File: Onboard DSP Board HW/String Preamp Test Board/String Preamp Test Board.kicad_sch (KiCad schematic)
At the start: 27 parts, among them J1 Battery, J4 Output Jack, U1 TLV9002, U2 TP4054, U6 ${SIM.PARAMS}

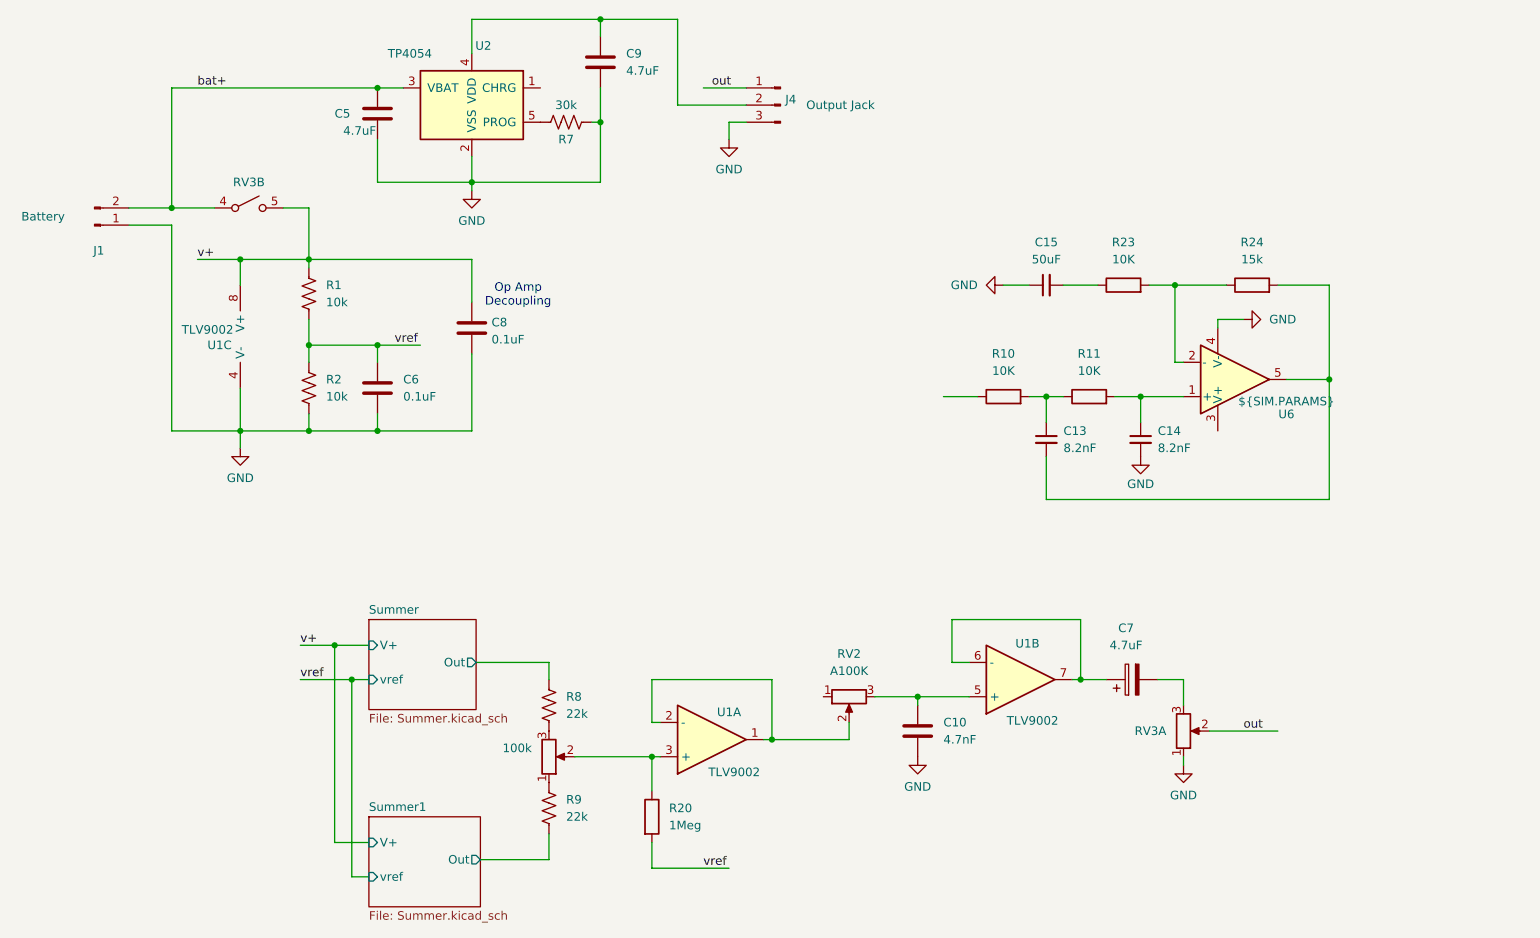
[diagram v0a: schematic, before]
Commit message: WIP
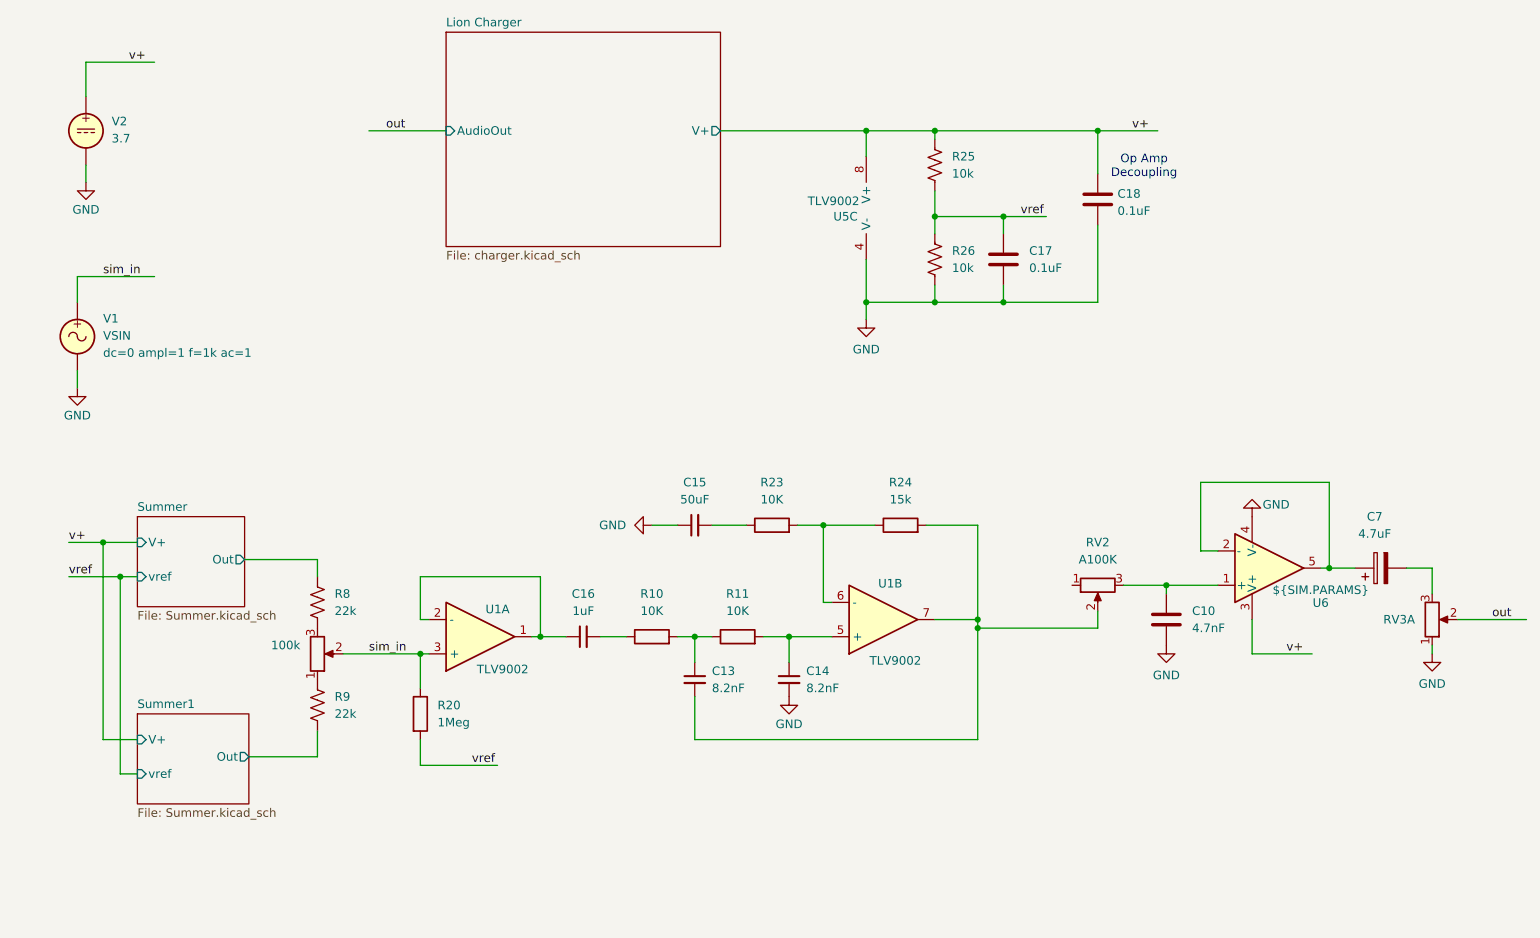
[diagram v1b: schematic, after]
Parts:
- removed C5, C9: 4.7uF, Capacitor_SMD:C_0603_1608Metric, symbol Device:C
- removed C6, C8: 0.1uF, Capacitor_SMD:C_0603_1608Metric, symbol Device:C
- removed J1: Battery, Connector_JST:JST_PH_S2B-PH-K_1x02_P2.00mm_Horizontal, symbol Connector:Conn_01x02_Male
- removed J4: Output Jack, Connector_PinHeader_2.54mm:PinHeader_1x03_P2.54mm_Vertical, symbol Connector:Conn_01x03_Male
- removed R1, R2: 10k, Resistor_SMD:R_0603_1608Metric, symbol Device:R_US
- removed R7: 30k, Resistor_SMD:R_0603_1608Metric, symbol Device:R_US
- removed unit 2 of RV3
- removed unit 3 of U1
- removed U2: TP4054, Package_TO_SOT_SMD:SOT-23-5, symbol Battery_Management:MCP73811T-420I-OT
- added C16: 1uF, symbol Device:C_Small
- added C17, C18: 0.1uF, Capacitor_SMD:C_0603_1608Metric, symbol Device:C
- added R25, R26: 10k, Resistor_SMD:R_0603_1608Metric, symbol Device:R_US
- added U5: TLV9002, Package_TO_SOT_SMD:SOT-23-8, symbol Amplifier_Operational:Opamp_Dual
- added V1: VSIN, symbol Simulation_SPICE:VSIN
- added V2: 3.7, symbol Simulation_SPICE:VDC
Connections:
- net GND: now also C17.1, C18.1, R26.1, U5.4 (V-), V1.2, V2.2
- net v+: now also U6.3 (V+), C18.2, R25.2, U5.8 (V+), V2.1
- net vref: now also C17.2, R25.1, R26.2
- net sim_in: now reaches R20.1, RV1.2, U1.3 (+)
- net sim_in: now also V1.1
- net at C13.2, R24.2: now also RV2.2, U1.7; no longer U6.5
- net at U1.1, U1.2 (-): now also C16.1; no longer RV2.2
- net at C10.2, RV2.3: now also U6.1 (+); no longer U1.5 (+)
- net at C14.1, R11.2: now also U1.5 (+); no longer U6.1 (+)
- net at R23.2, R24.1: now also U1.6 (-); no longer U6.2 (-)
- net at R10.1: now also C16.2
- new net: C7.1, U6.2 (-), U6.5
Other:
- added sheet Lion Charger (charger.kicad_sch)
- moved on the sheet: C10, C13, C14, C15, C7, R10, R11, R20, R23, R24, R8, R9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
